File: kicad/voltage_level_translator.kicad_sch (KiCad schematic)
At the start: 15 parts, among them Q1 2N7002, U3 TMUX1574PW, U7 TMUX1574PW, U8 TXS0108EPW, U9 TXS0108EPW

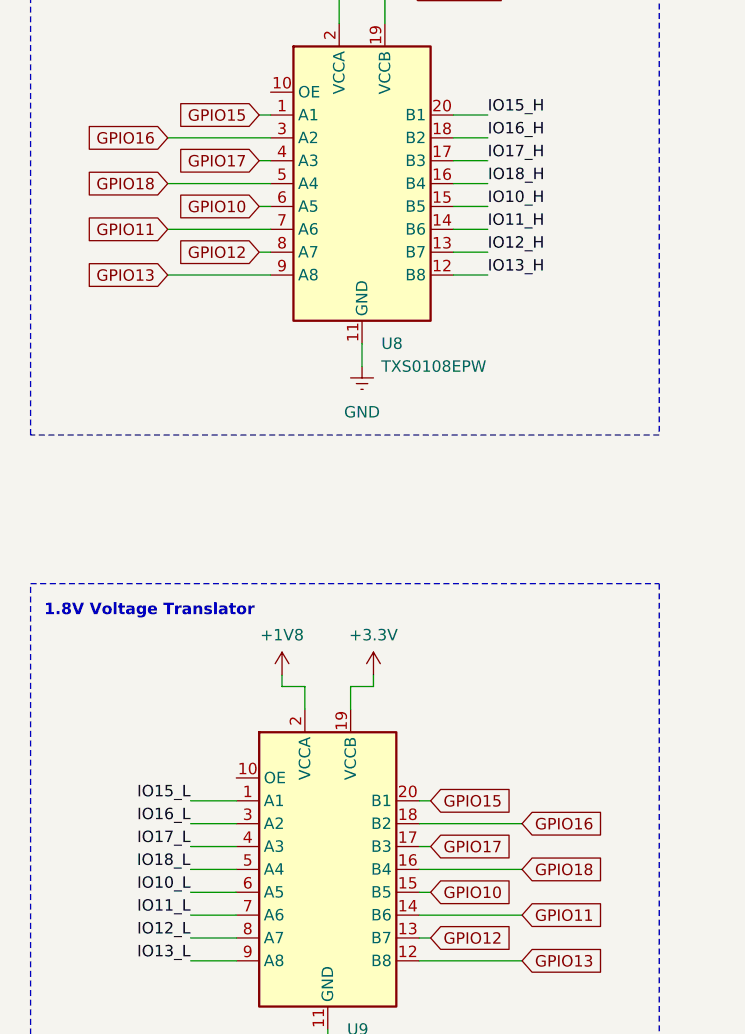
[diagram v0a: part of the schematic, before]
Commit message: Updated wiring
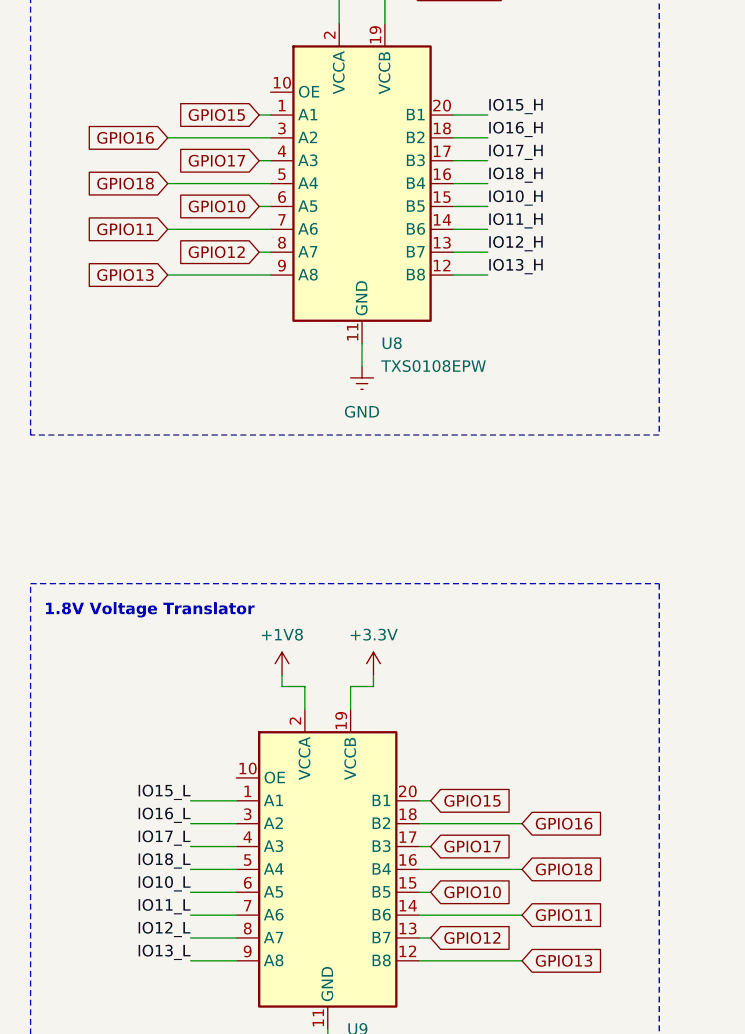
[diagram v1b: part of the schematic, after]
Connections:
- net IO18_H: now also U8.16 (B4)
- net IO18_L: now also U9.5 (A4)
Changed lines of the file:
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@@
+	(wire
+		(pts
+			(xy 36.83 127) (xy 41.91 127)
+		)
+		(stroke
+			(width 0)
+			(type default)
+		)
+	)
 	(wire
 		(pts
@@
 		(pts
 			(xy 231.14 30.48) (xy 232.41 30.48)
-		)
-		(stroke
-			(width 0)
-			(type default)
-		)
-	)
-	(wire
-		(pts
-			(xy 36.83 127) (xy 41.91 127)
 		)
 		(stroke
@@
 		)
 	)
-	(label "IO18_L"
-		(at 36.8095 127 180)
-		(effects
-			(font
-				(size 1.27 1.27)
-			)
-			(justify right bottom)
-		)
-	)
 	(label "IO13_H"
 		(at 266.7 135.89 0)
@@
 		)
 	)
+	(label "IO18_H"
+		(at 69.85 50.8 0)
+		(effects
+			(font
+				(size 1.27 1.27)
+			)
+			(justify left bottom)
+		)
+	)
 	(label "D1_K"
 		(at 140.97 74.93 0)
@@
 		)
 	)
-	(label "IO18_H"
-		(at 69.8705 50.8 0)
-		(effects
-			(font
-				(size 1.27 1.27)
-			)
-			(justify left bottom)
-		)
-	)
 	(label "IO11_H"
 		(at 69.85 55.88 0)
@@
 		)
 	)
+	(label "IO18_L"
+		(at 36.83 127 180)
+		(effects
+			(font
+				(size 1.27 1.27)
+			)
+			(justify right bottom)
+		)
+	)
